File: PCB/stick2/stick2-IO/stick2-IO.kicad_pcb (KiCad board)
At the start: 2 copper layers, 76 x 40.1 mm, 20 parts, among them J10 Conn_01x12_Pin, J11 Conn_01x04_Pin, J12 Conn_01x05_Pin, J13 Conn_01x16_Pin, J2 Conn_02x04_Row_Letter_Last, J3 Conn_02x04_Row_Letter_Last, J4 Conn_02x04_Row_Letter_Last, J5 Conn_02x04_Row_Letter_Last, J6 Conn_02x04_Row_Letter_Last, J7 Conn_02x04_Row_Letter_Last, J8 Conn_02x04_Row_Letter_Last, J9 Conn_02x04_Row_Letter_Last, U2 TLC5947RHB, U3 TLC5947RHB, U6 CD74HC4067M

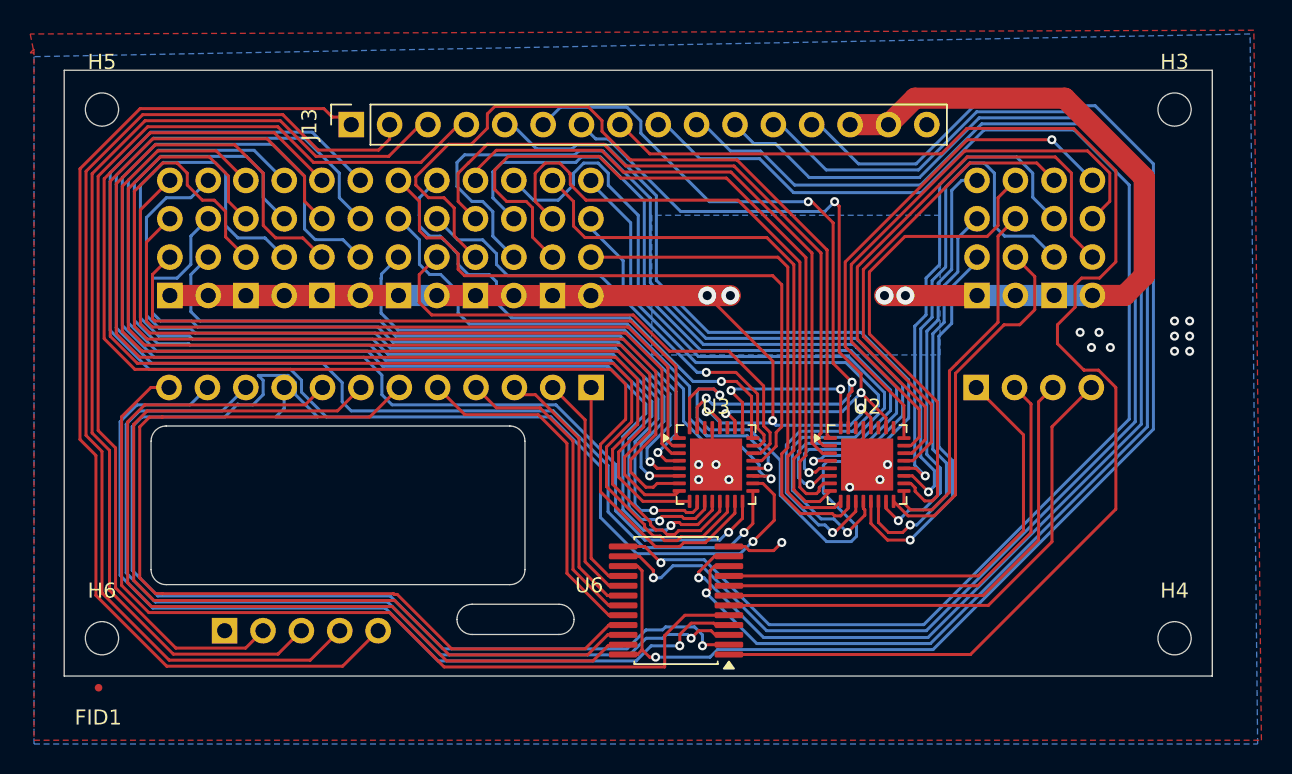
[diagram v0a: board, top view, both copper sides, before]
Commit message: board changes
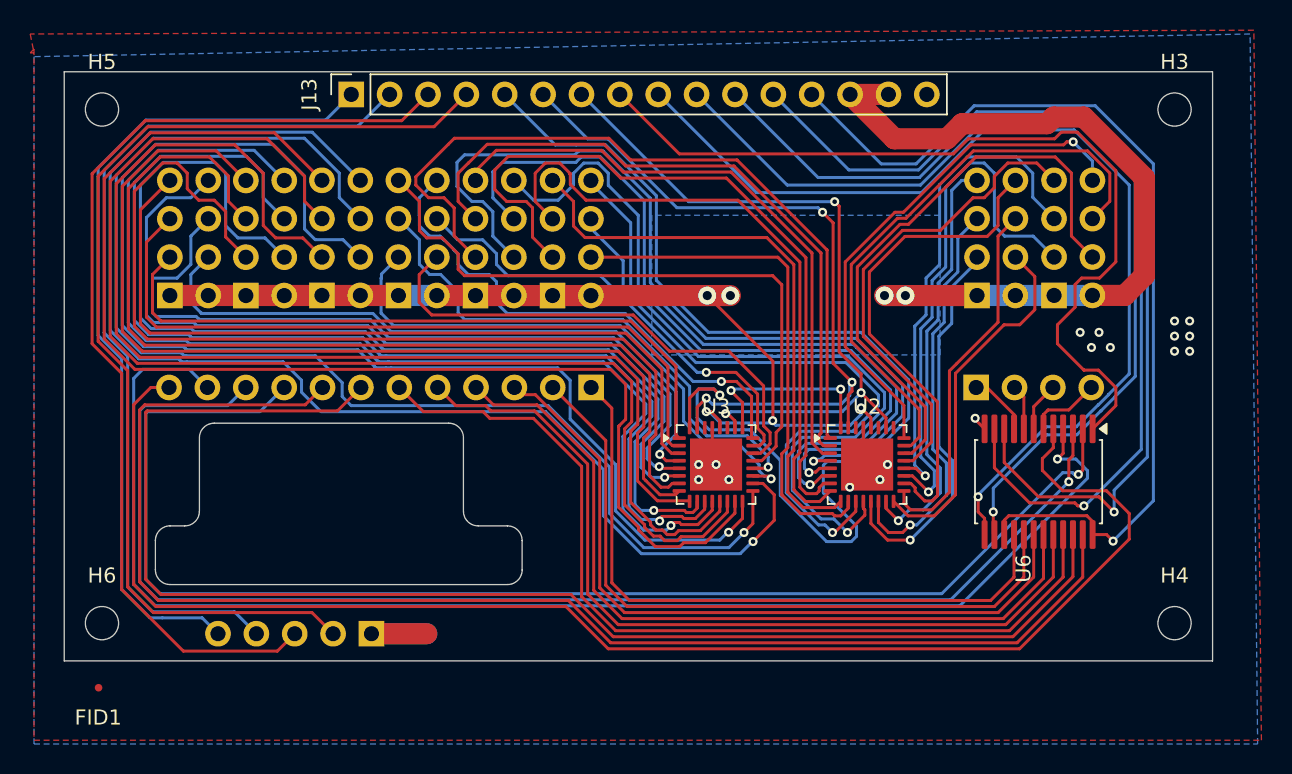
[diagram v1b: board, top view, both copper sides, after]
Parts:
- moved U6 25.3 mm to (164.0, 77.1), turned to -90 degrees
- moved J12 9.72 mm to (119.8, 87.2), turned to 90 degrees
- moved J13 2.00 mm to (118.5, 51.5)
- moved H4 1.00 mm to (173.0, 86.5)
- moved H6 1.00 mm to (102.0, 86.5)
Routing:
- net Net-(J10-Pin_12): track 60.2 -> 97.1 mm
- net /COM: track 92.0 -> 58.3 mm
- net Net-(J10-Pin_8): track 59.8 -> 92.8 mm
- net Net-(J10-Pin_5): track 23.6 -> 56.4 mm
- net Net-(J10-Pin_4): track 20.7 -> 52.9 mm
- net Net-(J10-Pin_7): track 61.4 -> 93.4 mm
- net Net-(J10-Pin_3): track 17.2 -> 48.7 mm
- net Net-(J10-Pin_2): track 15.6 -> 46.4 mm
- net Net-(J10-Pin_11): track 61.1 -> 91.4 mm
- net Net-(J10-Pin_1): track 13.9 -> 44.1 mm
- net /3.3v: track 92.9 -> 63.3 mm
- net Net-(J11-Pin_4): track 34.4 -> 4.85 mm
- net /S2: track 92.8 -> 63.2 mm
- net Net-(J11-Pin_3): track 32.5 -> 3.26 mm
- net Net-(J11-Pin_2): track 31.5 -> 2.99 mm
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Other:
- board size 76 x 40.1 mm -> 76 x 39 mm
